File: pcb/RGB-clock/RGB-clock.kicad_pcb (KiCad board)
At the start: 2 copper layers, 10 parts, among them P1 FTDI, P2 Display, SW1 Reset, SW2 Flash, U1 ESP-12

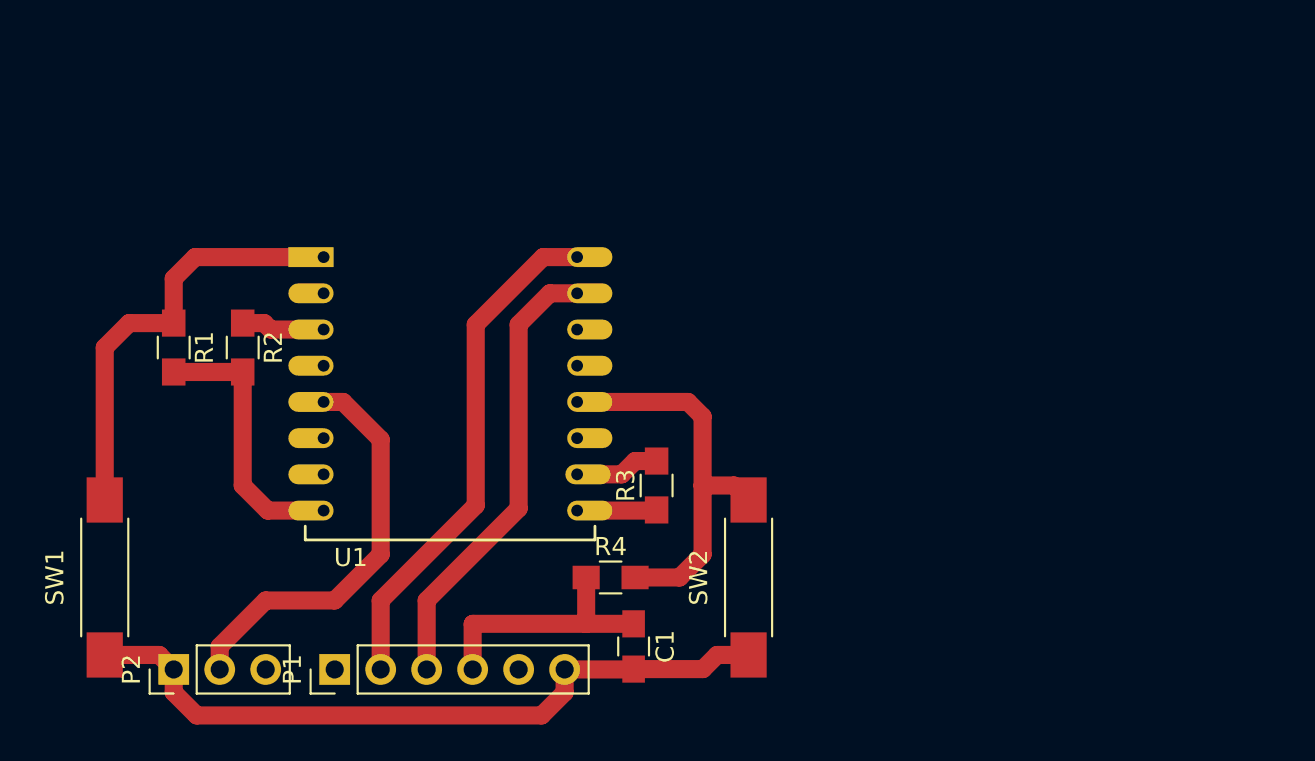
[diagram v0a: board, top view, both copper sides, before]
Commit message: Updated PCB
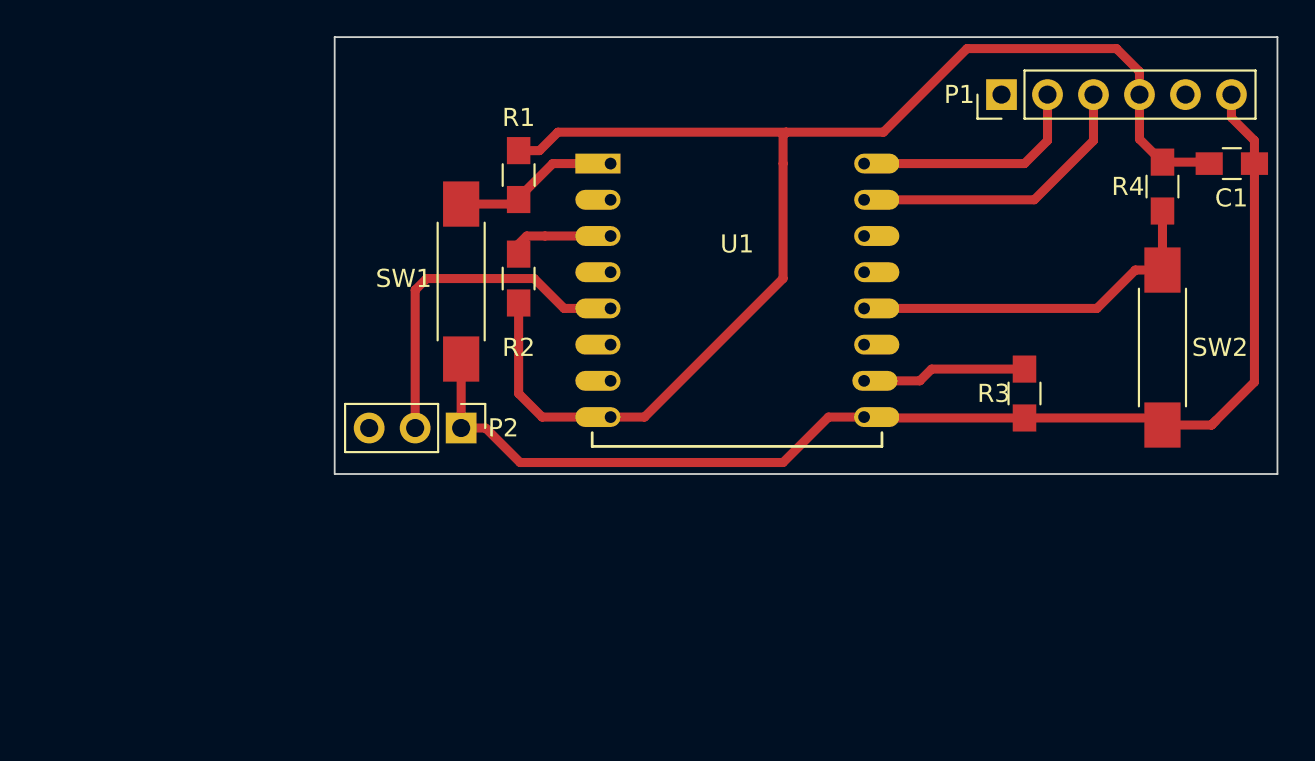
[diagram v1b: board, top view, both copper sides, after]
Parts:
- moved P1 48.6 mm to (162.6, 108.0)
- moved C1 42.5 mm to (175.3, 111.8), turned to 0 degrees
- moved R4 37.4 mm to (171.4, 113.0), turned to 270 degrees
- moved SW2 26.2 mm to (171.4, 121.9)
- moved SW1 25.6 mm to (132.7, 118.3)
- moved R1 21.3 mm to (135.9, 112.4), turned to 90 degrees
- moved R3 20.9 mm to (163.8, 124.5)
- moved P2 20.7 mm to (132.7, 126.4), turned to 270 degrees
- moved U1 16.7 mm to (141.0, 111.8)
- moved R2 15.7 mm to (135.9, 118.1)
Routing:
- net +3V3: track 29.1 -> 76.8 mm
- net GND: track 44.2 -> 67.4 mm
- net Net-(P1-Pad2): track 28.4 -> 13.2 mm
- net Net-(R1-Pad1): track 24.0 -> 9.24 mm
- net Net-(P1-Pad3): track 25.1 -> 16.6 mm
- net Net-(R3-Pad2): track 4.69 -> 9.13 mm
- net Net-(P2-Pad2): track 22.6 -> 19.4 mm
- net Net-(R4-Pad2): track 22.0 -> 20.6 mm
- net Net-(R2-Pad1): track 4.62 -> 5.82 mm
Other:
- board outline added: 52.1 x 24.1 mm
- net class Default: trace_width 1 -> 0.5
